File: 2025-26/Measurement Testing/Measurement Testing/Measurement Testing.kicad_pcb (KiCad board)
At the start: 2 copper layers, 75 x 75 mm, 21 parts, among them J1 Power Supply, J2 XT30PW-F, U1 TPS54308DDCR, U2 INA240A2PWR, U3 RASPBERRY_PI_PICO, U4 ADS8684IDBTR

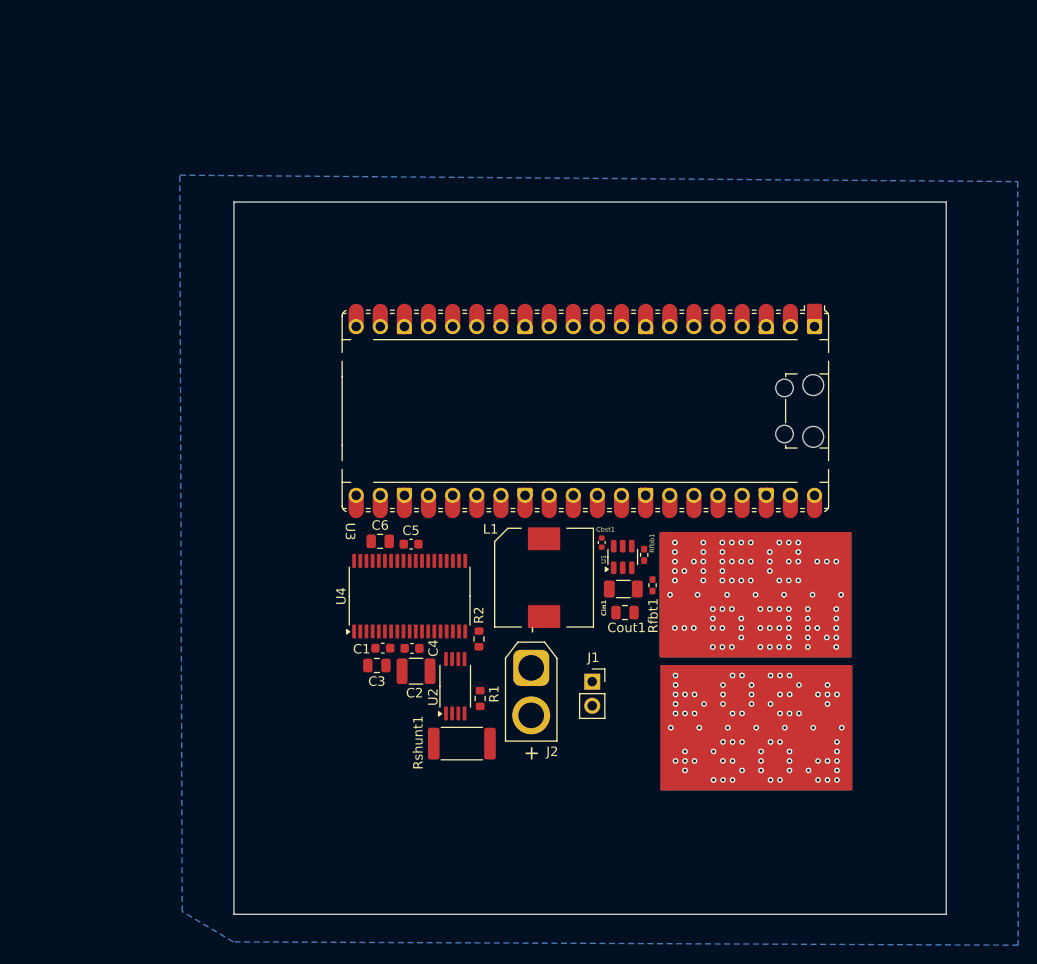
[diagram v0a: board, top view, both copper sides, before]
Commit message: basic layout done
yeah
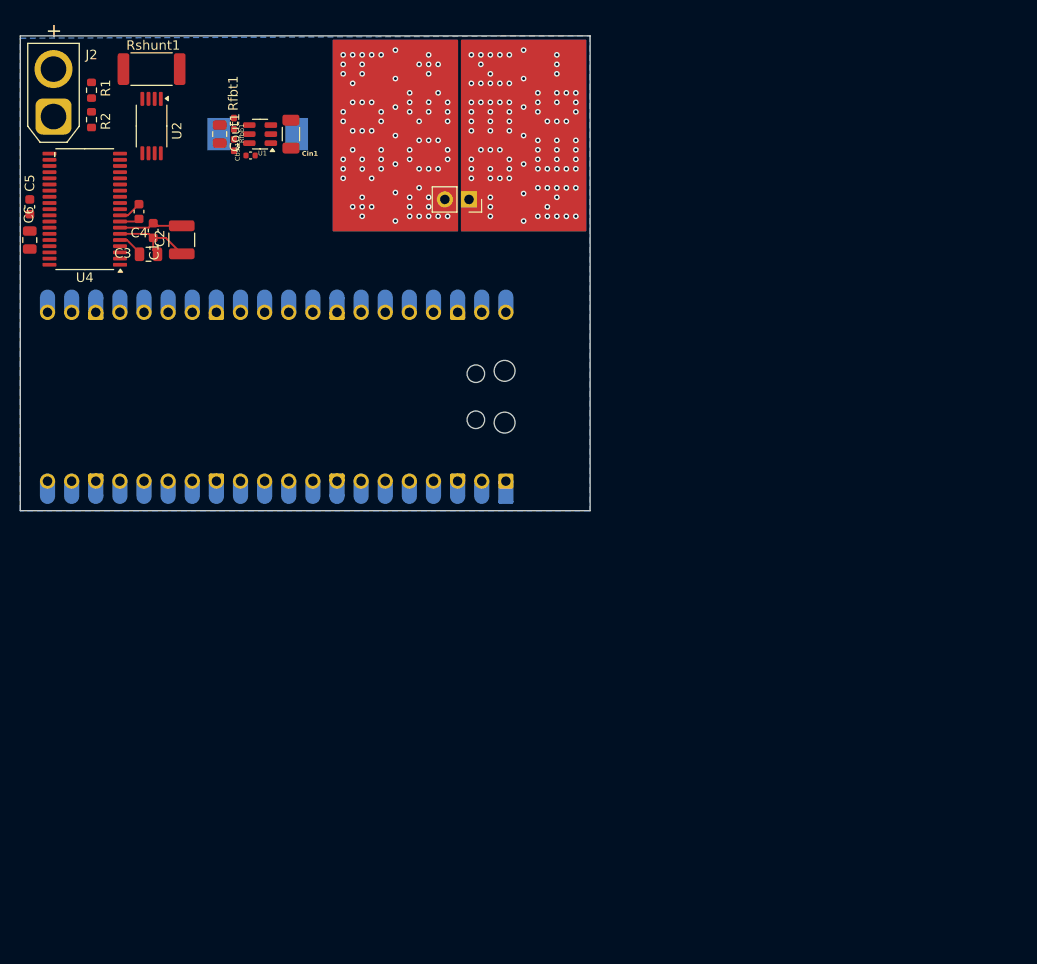
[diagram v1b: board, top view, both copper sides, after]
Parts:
- L1, U3: moved to B.Cu
- moved Rshunt1 78.2 mm to (83.8, 28.5), turned to 180 degrees
- moved J2 76.8 mm to (73.5, 33.5), turned to 90 degrees
- moved R1 76.0 mm to (77.5, 30.7), turned to -90 degrees
- moved R2 68.2 mm to (77.5, 33.8), turned to -90 degrees
- moved U2 67.1 mm to (83.8, 34.5), turned to -90 degrees
- moved Cout1 66.0 mm to (91.0, 35.3), turned to -90 degrees
- moved Rfbt1 65.6 mm to (92.5, 34.2), turned to -90 degrees
- moved Rfbb1 61.1 mm to (92.5, 36.5)
- moved Cin1 59.3 mm to (98.5, 35.3), turned to -90 degrees
- moved U1 58.7 mm to (95.2, 35.3), turned to 180 degrees
- moved L1 55.6 mm to (95.0, 35.3), turned to 180 degrees
- moved Cbst1 55.0 mm to (94.2, 37.6), turned to 0 degrees
- moved C4 54.2 mm to (82.5, 43.5), turned to -90 degrees
- moved C5 53.6 mm to (71.0, 43.0), turned to 90 degrees
- moved U4 53.2 mm to (76.8, 43.2), turned to 180 degrees
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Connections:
- Cout1 pad 1: /5V_PSU/Iout -> 5V
- L1 pad 2: /5V_PSU/Iout -> 5V
- Rfbt1 pad 1: /5V_PSU/Iout -> 5V
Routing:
- net GND: track 0.00 -> 11.4 mm
- net Net-(U4-REFCAP): track 0.00 -> 6.81 mm
- net Net-(U4-REFIO): track 0.00 -> 2.78 mm
- net 5V: track 0.00 -> 2.49 mm
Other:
- board size 75 x 75 mm -> 60 x 50 mm
